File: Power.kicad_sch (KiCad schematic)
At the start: 38 parts, among them IC1 LM66200DRLR, J22 Conn_01x02, U10 LP2985-3.3, U9 AP63203WU

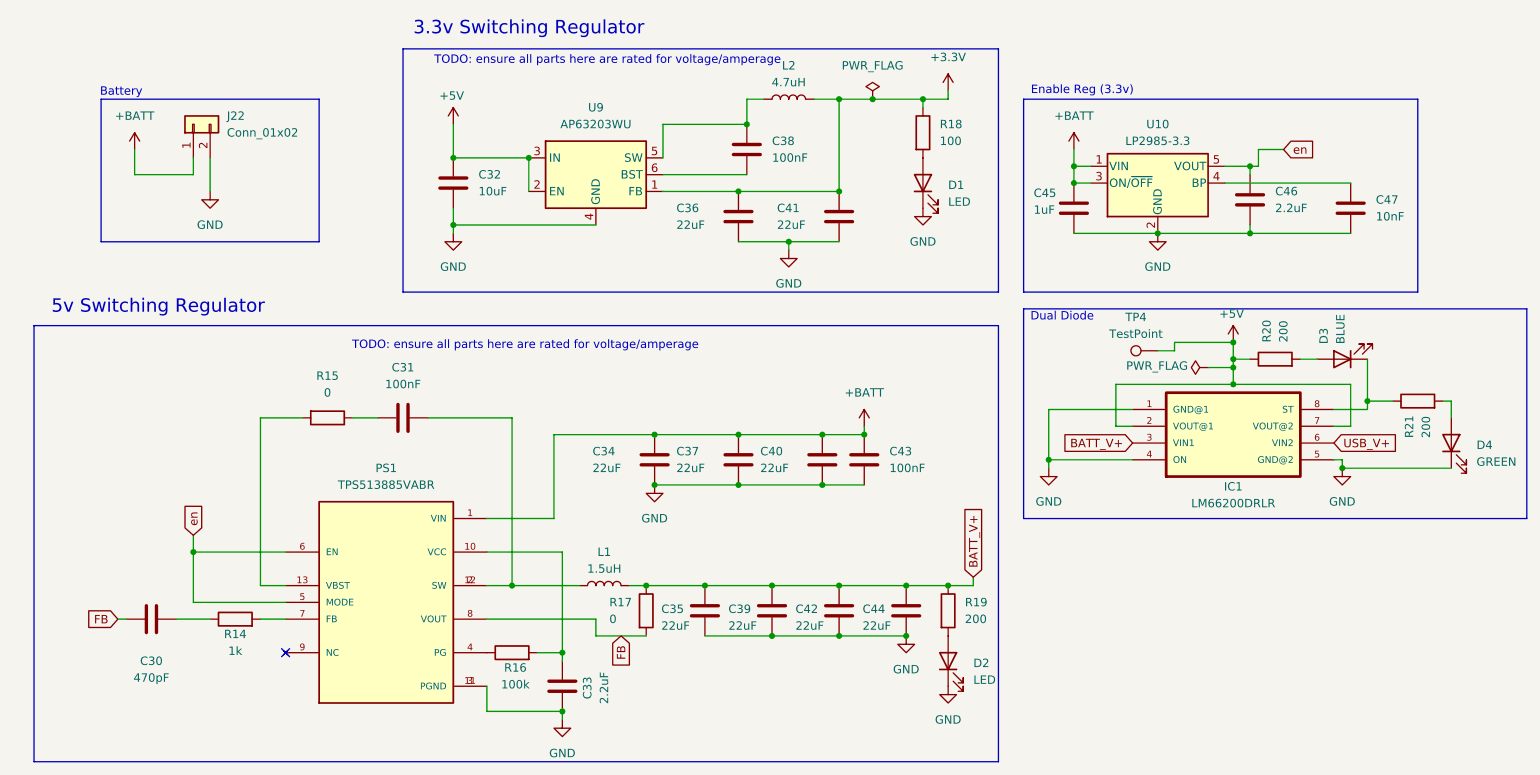
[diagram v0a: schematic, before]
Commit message: First Draft of BOM
Didn't select some compoentns like diodes that I don't fully understand. Also, some components have multiple variants so we must be careful.
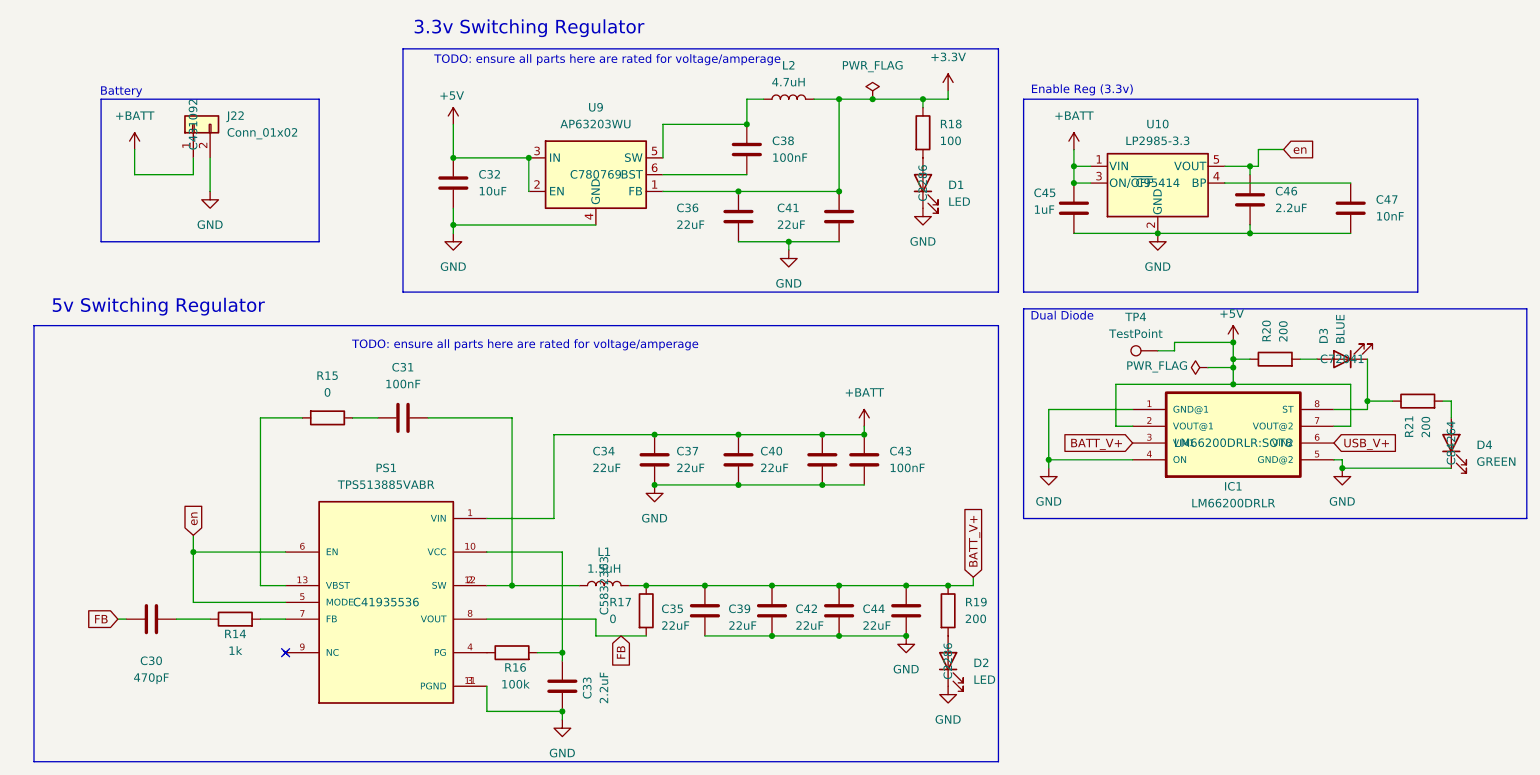
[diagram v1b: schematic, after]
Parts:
- D1, D2: JLC# (none) -> C2286
- D3: JLC# (none) -> C72041
- D4: JLC# (none) -> C84264
- IC1: JLC# (none) -> LM66200DRLR:SOT8
- J22: JLC# (none) -> C431092
- L1: JLC# (none) -> C5832363
- PS1: JLC# (none) -> C41935536
- U10: JLC# (none) -> C95414
- U9: JLC# (none) -> C780769

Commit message: parts⚙️
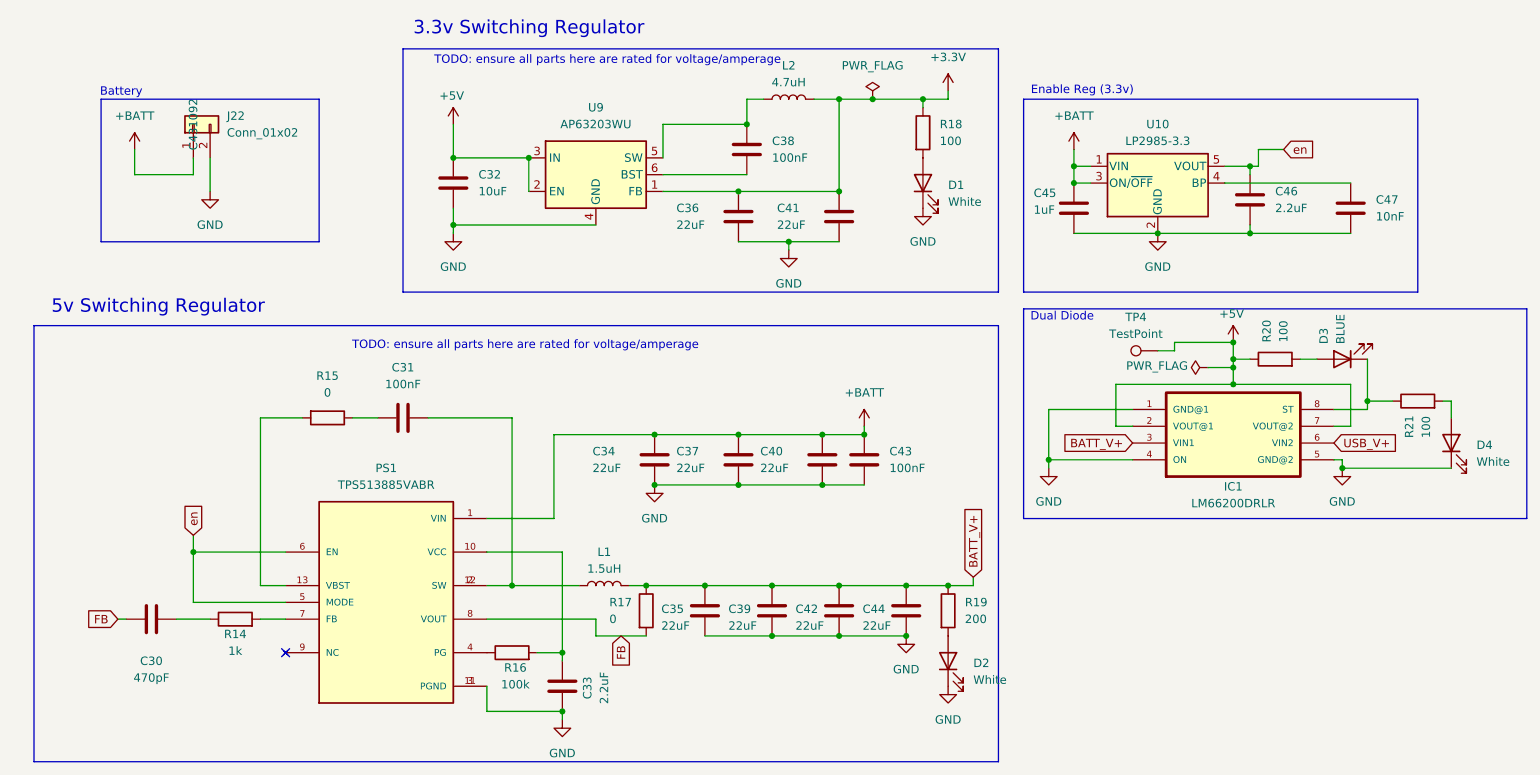
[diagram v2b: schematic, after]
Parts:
- D1, D2: value LED -> White; JLC# C2286 -> C965808
- D3: JLC# C72041 -> C965807
- D4: value GREEN -> White; JLC# C84264 -> C965808
- IC1: JLC# LM66200DRLR:SOT8 -> C3235556
- L1: footprint Inductor_SMD:L_1008_2520Metric -> CYA0630-1.5UH:IND_CYA0630_SHH; JLC# C5832363 -> C5189745
- L2: footprint Inductor_SMD:L_1008_2520Metric -> Inductor_SMD:L_Changjiang_FNR4030S; JLC# (none) -> C167874
- R20, R21: value 200 -> 100
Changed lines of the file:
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@@
 			)
 		)
-		(property "Footprint" "Inductor_SMD:L_1008_2520Metric"
+		(property "Footprint" "Inductor_SMD:L_Changjiang_FNR4030S"
 			(at 138.43 66.04 0)
 			(effects
@@
 			)
 		)
-		(property "JLC#" ""
+		(property "JLC#" "C167874"
 			(at 138.43 66.04 0)
 			(effects
@@
 					(size 1.27 1.27)
 				)
+				(hide yes)
 			)
 		)
@@
 			)
 		)
-		(property "Value" "LED"
+		(property "Value" "White"
 			(at 166.37 153.9874 90)
 			(effects
@@
 			)
 		)
-		(property "JLC#" "C2286"
+		(property "JLC#" "C965808"
 			(at 162.56 151.13 0)
 			(effects
@@
 					(size 1.27 1.27)
 				)
+				(hide yes)
 			)
 		)
@@
 					(size 1.27 1.27)
 				)
+				(hide yes)
 			)
 		)
@@
 			)
 		)
-		(property "Footprint" "Inductor_SMD:L_1008_2520Metric"
+		(property "Footprint" "CYA0630-1.5UH:IND_CYA0630_SHH"
 			(at 110.49 139.7 0)
 			(effects
@@
 			)
 		)
-		(property "JLC#" "C5832363"
+		(property "JLC#" "C5189745 "
 			(at 110.49 139.7 0)
 			(effects
@@
 					(size 1.27 1.27)
 				)
+				(hide yes)
 			)
 		)
@@
 			)
 		)
-		(property "Value" "LED"
+		(property "Value" "White"
 			(at 162.56 81.5974 90)
 			(effects
@@
 			)
 		)
-		(property "JLC#" "C2286"
+		(property "JLC#" "C965808"
 			(at 158.75 78.74 0)
 			(effects
@@
 					(size 1.27 1.27)
 				)
+				(hide yes)
 			)
 		)
@@
 					(size 1.27 1.27)
 				)
+				(hide yes)
 			)
 		)
@@
 			)
 		)
-		(property "Value" "GREEN"
+		(property "Value" "White"
 			(at 242.57 120.9674 90)
 			(effects
@@
 			)
 		)
-		(property "JLC#" "C84264"
+		(property "JLC#" "C965808"
 			(at 238.76 118.11 0)
 			(effects
@@
 					(size 1.27 1.27)
 				)
+				(hide yes)
 			)
 		)
@@
 					(size 1.27 1.27)
 				)
+				(hide yes)
 			)
 		)
@@
 			)
 		)
-		(property "Value" "200"
+		(property "Value" "100"
 			(at 213.3599 102.87 0)
 			(effects
@@
 			)
 		)
-		(property "JLC#" "C72041"
+		(property "JLC#" "C965807"
 			(at 222.25 105.41 0)
 			(effects
@@
 					(size 1.27 1.27)
 				)
+				(hide yes)
 			)
 		)
@@
 			)
 		)
-		(property "Value" "200"
+		(property "Value" "100"
 			(at 234.95 117.348 0)
 			(effects
@@
 			)
 		)
-		(property "JLC#" "LM66200DRLR:SOT8"
+		(property "JLC#" "C3235556"
 			(at 205.74 118.11 0)
 			(effects
@@
 					(size 1.27 1.27)
 				)
+				(hide yes)
 			)
 		)

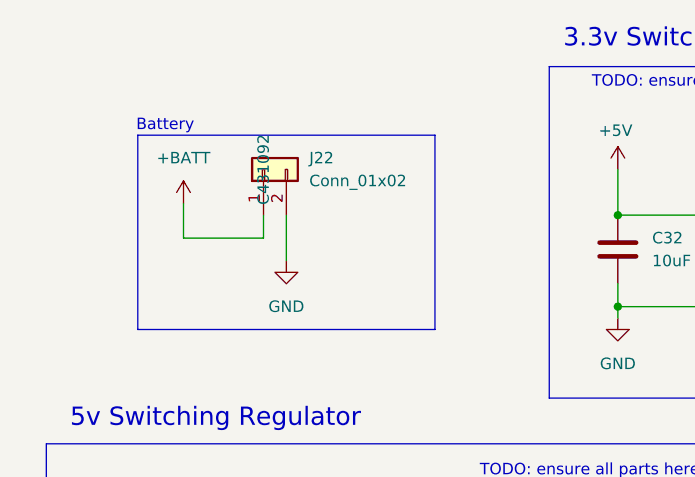
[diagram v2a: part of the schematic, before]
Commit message: ⚡️⚙️🐘😂
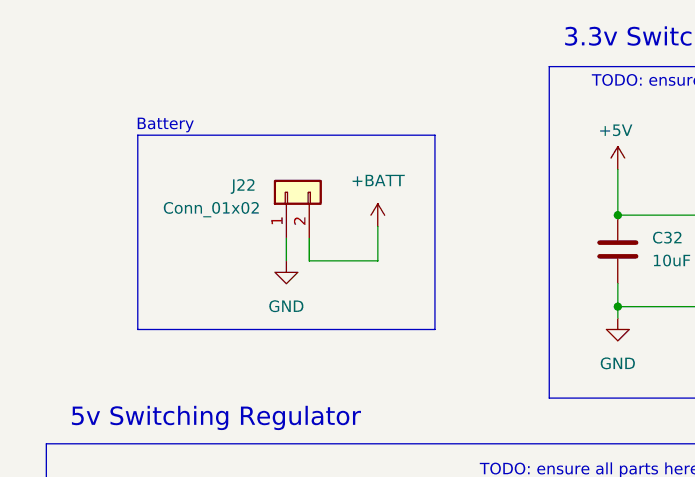
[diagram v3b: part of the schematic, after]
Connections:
- net +BATT: now also J22.2 (Pin_2); no longer J22.1 (Pin_1)
- net GND: now also J22.1 (Pin_1); no longer J22.2 (Pin_2)
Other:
- moved on the sheet: J22
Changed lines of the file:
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@@
 	(wire
 		(pts
-			(xy 39.37 77.47) (xy 48.26 77.47)
+			(xy 72.39 114.3) (xy 76.2 114.3)
 		)
 		(stroke
@@
 	(wire
 		(pts
-			(xy 72.39 114.3) (xy 76.2 114.3)
+			(xy 146.05 80.01) (xy 146.05 66.04)
 		)
 		(stroke
@@
 	(wire
 		(pts
-			(xy 146.05 80.01) (xy 146.05 66.04)
+			(xy 60.96 80.01) (xy 60.96 76.2)
 		)
 		(stroke
@@
 	(wire
 		(pts
-			(xy 39.37 73.66) (xy 39.37 77.47)
-		)
-		(stroke
-			(width 0)
-			(type default)
-		)
-	)
-	(wire
-		(pts
 			(xy 166.37 138.43) (xy 166.37 139.7)
 		)
@@
 	(wire
 		(pts
+			(xy 53.34 77.47) (xy 53.34 80.01)
+		)
+		(stroke
+			(width 0)
+			(type default)
+		)
+	)
+	(wire
+		(pts
 			(xy 102.87 116.84) (xy 102.87 129.54)
 		)
@@
 	(wire
 		(pts
-			(xy 48.26 77.47) (xy 48.26 74.93)
+			(xy 50.8 80.01) (xy 50.8 77.47)
 		)
 		(stroke
@@
 	(wire
 		(pts
-			(xy 50.8 80.01) (xy 50.8 74.93)
-		)
-		(stroke
-			(width 0)
-			(type default)
-		)
-	)
-	(wire
-		(pts
 			(xy 146.05 66.04) (xy 151.13 66.04)
 		)
@@
 	(wire
 		(pts
+			(xy 53.34 80.01) (xy 60.96 80.01)
+		)
+		(stroke
+			(width 0)
+			(type default)
+		)
+	)
+	(wire
+		(pts
 			(xy 181.61 76.2) (xy 184.15 76.2)
 		)
@@
 	(symbol
 		(lib_id "Connector_Generic:Conn_01x02")
-		(at 48.26 69.85 90)
+		(at 50.8 72.39 90)
 		(unit 1)
 		(exclude_from_sim no)
@@
 		(on_board yes)
 		(dnp no)
-		(fields_autoplaced yes)
 		(property "Reference" "J22"
-			(at 53.34 68.5799 90)
+			(at 44.704 71.628 90)
 			(effects
 				(font
@@
 		)
 		(property "Value" "Conn_01x02"
-			(at 53.34 71.1199 90)
+			(at 37.084 74.168 90)
 			(effects
 				(font
@@
 		)
 		(property "Footprint" "Connector_AMASS:AMASS_XT30PW-M_1x02_P2.50mm_Horizontal"
-			(at 48.26 69.85 0)
+			(at 50.8 72.39 0)
 			(effects
 				(font
@@
 		)
 		(property "Datasheet" "~"
-			(at 48.26 69.85 0)
+			(at 50.8 72.39 0)
 			(effects
 				(font
@@
 		)
 		(property "Description" "Generic connector, single row, 01x02, script generated (kicad-library-utils/schlib/autogen/connector/)"
-			(at 48.26 69.85 0)
+			(at 50.8 72.39 0)
 			(effects
 				(font
@@
 		)
 		(property "JLC#" "C431092"
-			(at 48.26 69.85 0)
+			(at 50.8 72.39 0)
 			(effects
 				(font
 					(size 1.27 1.27)
 				)
+				(hide yes)
 			)
 		)
@@
 	(symbol
 		(lib_id "power:+BATT")
-		(at 39.37 73.66 0)
+		(at 60.96 76.2 0)
 		(unit 1)
 		(exclude_from_sim no)
@@
 		(fields_autoplaced yes)
 		(property "Reference" "#PWR078"
-			(at 39.37 77.47 0)
+			(at 60.96 80.01 0)
 			(effects
 				(font
@@
 		)
 		(property "Value" "+BATT"
-			(at 39.37 68.58 0)
+			(at 60.96 71.12 0)
 			(effects
 				(font
@@
 		)
 		(property "Footprint" ""
-			(at 39.37 73.66 0)
+			(at 60.96 76.2 0)
 			(effects
 				(font
@@
 		)
 		(property "Datasheet" ""
-			(at 39.37 73.66 0)
+			(at 60.96 76.2 0)
 			(effects
 				(font
@@
 		)
 		(property "Description" "Power symbol creates a global label with name \"+BATT\""
-			(at 39.37 73.66 0)
+			(at 60.96 76.2 0)
 			(effects
 				(font
